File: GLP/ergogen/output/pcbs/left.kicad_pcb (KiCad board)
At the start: 2 copper layers, 138.8 x 106.7 mm, 66 parts

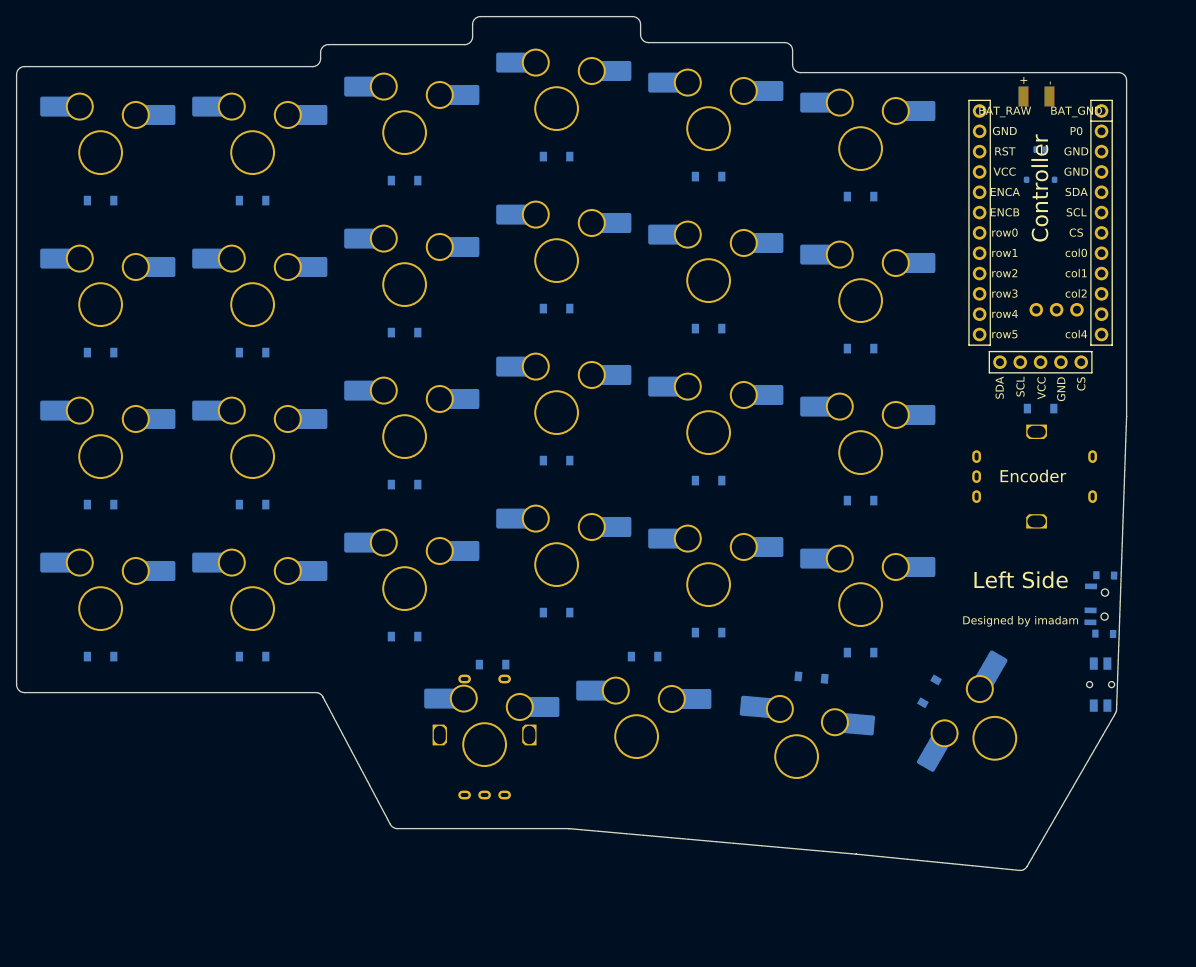
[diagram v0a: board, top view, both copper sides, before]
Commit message: er i lied
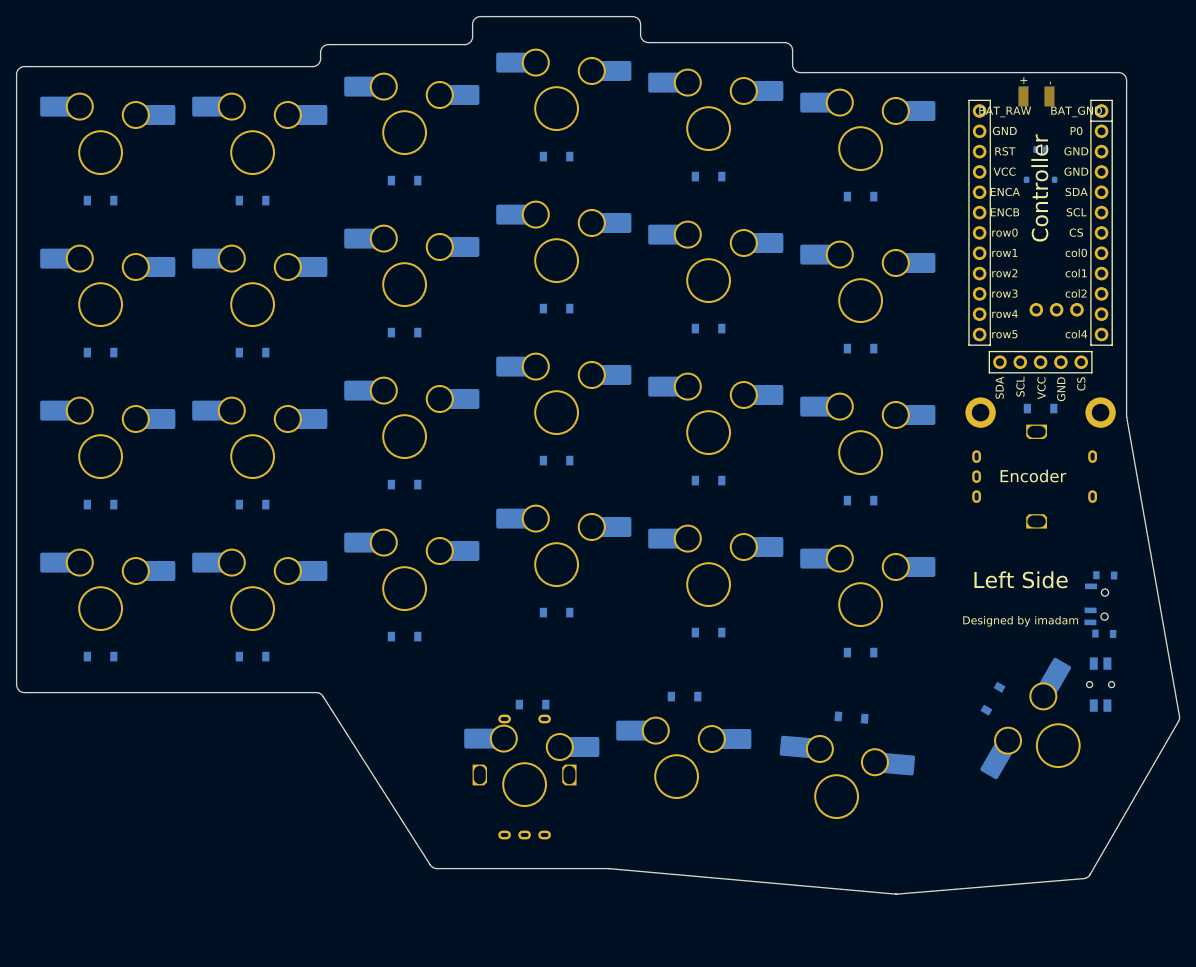
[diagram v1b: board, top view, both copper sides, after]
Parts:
- added H1: , ceoloide:mounting_hole_plated, F.Cu at (160.0, 106.5)
- added H2: , ceoloide:mounting_hole_plated, F.Cu at (175.0, 106.5)
- moved D28 7.99 mm to (161.6, 142.3)
- moved S28 7.99 mm to (169.7, 148.1)
- moved D25 7.07 mm to (104.0, 143.0)
- moved D26 7.07 mm to (123.0, 142.0)
- moved D27 7.07 mm to (143.9, 144.6)
- moved RE2 7.07 mm to (103.0, 151.8)
- moved S25 7.07 mm to (103.0, 153.0)
- moved S26 7.07 mm to (122.0, 152.0)
- moved S27 7.07 mm to (142.0, 154.5)
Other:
- board size 138.8 x 106.7 mm -> 145.4 x 109.7 mm
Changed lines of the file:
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@@
   (title_block
     (title "left")
-    (date "2025-04-06")
+    (date "2025-04-07")
     (rev "v1.0.0")
     (company "Unknown")
@@
   (footprint "ceoloide:switch_gateron_ks27_ks33"
     (layer "B.Cu")
-    (at 98 148 180)
+    (at 103 153 180)
     (property "Reference" "S25"
       (at 0 8.8 180)
@@
   (footprint "ceoloide:switch_gateron_ks27_ks33"
     (layer "B.Cu")
-    (at 117 147 180)
+    (at 122 152 180)
     (property "Reference" "S26"
       (at 0 8.8 180)
@@
   (footprint "ceoloide:switch_gateron_ks27_ks33"
     (layer "B.Cu")
-    (at 137 149.5 175)
+    (at 142 154.5 175)
     (property "Reference" "S27"
       (at 0 8.8 175)
@@
   (footprint "ceoloide:switch_gateron_ks27_ks33"
     (layer "B.Cu")
-    (at 161.777353 147.2132953 240)
+    (at 169.71036569999998 148.1331683 240)
     (property "Reference" "S28"
       (at 0 8.8 240)
@@
     (footprint "ceoloide:diode_tht_sod123"
         (layer "B.Cu")
-        (at 99 138 0)
+        (at 104 143 0)
         (property "Reference" "D25"
             (at 0 0 0)
@@
     (footprint "ceoloide:diode_tht_sod123"
         (layer "B.Cu")
-        (at 118 137 0)
+        (at 123 142 0)
         (property "Reference" "D26"
             (at 0 0 0)
@@
     (footprint "ceoloide:diode_tht_sod123"
         (layer "B.Cu")
-        (at 138.8677521 139.6252088 -5)
+        (at 143.8677521 144.6252088 -5)
         (property "Reference" "D27"
             (at 0 0 -5)
@@
     (footprint "ceoloide:diode_tht_sod123"
         (layer "B.Cu")
-        (at 153.617099 141.3472699 60)
+        (at 161.55011169999997 142.26714289999998 60)
         (property "Reference" "D28"
             (at 0 0 60)
@@
   (footprint "ceoloide:rotary_encoder_ec11_ec12"
     (layer "F.Cu")
-    (at 98 146.8 0)
+    (at 103 151.8 0)
     (property "Reference" "RE2"
       (at 0 -8.5)
@@
   )
   (gr_text "Bottom"
-    (at 136.4770655 155.4771682 -5)
+    (at 141.4770655 160.4771682 -5)
     (layer "B.SilkS" knockout)
     (effects
@@
       )
     )
+  )
+  (footprint "ceoloide:mounting_hole_plated"
+    (layer "F.Cu")
+    (at 160 106.5 0)
+    (property "Reference" "H1"
+      (at 0 3 0)
+      (layer "F.SilkS")
+      hide
+      (effects (font (size 1 1) (thickness 0.15)))
+    )
+    (pad "" thru_hole circle (at 0 0 0) (size 3.8000000000000003 3.8000000000000003) (drill 2.2) (layers "*.Cu" "*.Mask"))
+    (fp_circle (center 0 0) (end -2.1500000000000004 0) (layer "F.CrtYd") (stroke (width 0.05) (type solid)) (fill none))
+    (fp_circle (center 0 0) (end -2.1500000000000004 0) (layer "B.CrtYd") (stroke (width 0.05) (type solid)) (fill none))
+  )
+  (footprint "ceoloide:mounting_hole_plated"
+    (layer "F.Cu")
+    (at 175 106.5 0)
+    (property "Reference" "H2"
+      (at 0 3 0)
+      (layer "F.SilkS")
+      hide
+      (effects (font (size 1 1) (thickness 0.15)))
+    )
+    (pad "" thru_hole circle (at 0 0 0) (size 3.8000000000000003 3.8000000000000003) (drill 2.2) (layers "*.Cu" "*.Mask"))
+    (fp_circle (center 0 0) (end -2.1500000000000004 0) (layer "F.CrtYd") (stroke (width 0.05) (type solid)) (fill none))
+    (fp_circle (center 0 0) (end -2.1500000000000004 0) (layer "B.CrtYd") (stroke (width 0.05) (type solid)) (fill none))
   )
   (gr_line (start 39.5 140.51) (end 39.5 64.24) (layer Edge.Cuts) (stroke (width 0.15) (type default)))
@@
 (gr_line (start 136.5 61.24) (end 136.5 63.01) (layer Edge.Cuts) (stroke (width 0.15) (type default)))
 (gr_line (start 137.49 64) (end 177.26 64) (layer Edge.Cuts) (stroke (width 0.15) (type default)))
-(gr_line (start 178.25 106.98304477713282) (end 178.25 64.99) (layer Edge.Cuts) (stroke (width 0.15) (type default)))
-(gr_line (start 178.249419298365 107.01694732484975) (end 176.99510974489652 143.62299453267315) (layer Edge.Cuts) (stroke (width 0.15) (type default)))
-(gr_line (start 176.86305555803136 144.08409196503845) (end 165.80615268800693 163.23520942658655) (layer Edge.Cuts) (stroke (width 0.15) (type default)))
-(gr_line (start 164.85076974921034 163.7253452437892) (end 144.47054179145226 161.6975779835782) (layer Edge.Cuts) (stroke (width 0.15) (type default)))
-(gr_line (start 144.46018222869026 161.69660218659897) (end 108.54374262754885 158.5038884057367) (layer Edge.Cuts) (stroke (width 0.15) (type default)))
-(gr_line (start 87.09606054117646 158.5) (end 108.45608436301427 158.5) (layer Edge.Cuts) (stroke (width 0.15) (type default)))
-(gr_line (start 86.22111054608999 157.9732088092811) (end 77.77888945391003 142.02679119071894) (layer Edge.Cuts) (stroke (width 0.15) (type default)))
-(gr_line (start 40.49 141.5) (end 76.90393945882354 141.5) (layer Edge.Cuts) (stroke (width 0.15) (type default)))
+(gr_line (start 178.25 106.91330563065048) (end 178.25 64.99) (layer Edge.Cuts) (stroke (width 0.15) (type default)))
+(gr_line (start 178.26506800524558 107.08537446037167) (end 184.85701419664065 144.43496650770498) (layer Edge.Cuts) (stroke (width 0.15) (type default)))
+(gr_line (start 184.73944731338625 145.10203531750773) (end 173.67873709901966 164.25974729286952) (layer Edge.Cuts) (stroke (width 0.15) (type default)))
+(gr_line (start 172.90327558014778 164.75135351340012) (end 149.55016624203031 166.69002289360108) (layer Edge.Cuts) (stroke (width 0.15) (type default)))
+(gr_line (start 149.3806043848676 166.68952828725241) (end 113.54374262754898 163.5038884057367) (layer Edge.Cuts) (stroke (width 0.15) (type default)))
+(gr_line (start 92.04345643636363 163.5) (end 113.4560843630144 163.5) (layer Edge.Cuts) (stroke (width 0.15) (type default)))
+(gr_line (start 91.20823156106951 163.04150673882353) (end 77.7917684389305 141.9584932611765) (layer Edge.Cuts) (stroke (width 0.15) (type default)))
+(gr_line (start 40.49 141.5) (end 76.95654356363637 141.5) (layer Edge.Cuts) (stroke (width 0.15) (type default)))
 (gr_arc (start 40.49 63.24999999999999) (mid 39.7899643 63.539964299999994) (end 39.5 64.24) (layer Edge.Cuts) (stroke (width 0.15) (type default)))
 (gr_arc (start 76.51 63.25) (mid 77.2100357 62.9600357) (end 77.5 62.26) (layer Edge.Cuts) (stroke (width 0.15) (type default)))
@@
 (gr_arc (start 136.5 63.01) (mid 136.7899643 63.7100357) (end 137.49 64) (layer Edge.Cuts) (stroke (width 0.15) (type default)))
 (gr_arc (start 178.25 64.99) (mid 177.9600357 64.2899643) (end 177.26 63.99999999999999) (layer Edge.Cuts) (stroke (width 0.15) (type default)))
-(gr_arc (start 178.2494193 107.01694727713281) (mid 178.24985479999998 106.99999847713282) (end 178.25 106.98304477713282) (layer Edge.Cuts) (stroke (width 0.15) (type default)))
-(gr_arc (start 176.8630555465315 144.08409198495713) (mid 176.9574287465315 143.86166138495713) (end 176.9951097465315 143.62299458495713) (layer Edge.Cuts) (stroke (width 0.15) (type default)))
-(gr_arc (start 164.8507697765069 163.7253452465051) (mid 165.4006839765069 163.6210554465051) (end 165.8061527765069 163.2352094465051) (layer Edge.Cuts) (stroke (width 0.15) (type default)))
-(gr_arc (start 144.47054176415568 161.6975779808623) (mid 144.46536326415568 161.69707648086228) (end 144.46018216415567 161.6966021808623) (layer Edge.Cuts) (stroke (width 0.15) (type default)))
-(gr_arc (start 108.54374266301427 158.50388840000002) (mid 108.49995666301427 158.5009726) (end 108.45608436301427 158.5) (layer Edge.Cuts) (stroke (width 0.15) (type default)))
-(gr_arc (start 86.22111054117646 157.97320879999998) (mid 86.58541234117645 158.3581381) (end 87.09606054117646 158.49999989999998) (layer Edge.Cuts) (stroke (width 0.15) (type default)))
-(gr_arc (start 77.77888945882354 142.02679120000002) (mid 77.41458765882355 141.6418619) (end 76.90393945882354 141.50000010000002) (layer Edge.Cuts) (stroke (width 0.15) (type default)))
+(gr_arc (start 178.25 106.91330563065048) (mid 178.2537742 106.99966933065049) (end 178.265068 107.08537443065049) (layer Edge.Cuts) (stroke (width 0.15) (type default)))
+(gr_arc (start 184.73944730188623 145.1020353374263) (mid 184.85705570188622 144.77886843742627) (end 184.85701410188622 144.43496653742628) (layer Edge.Cuts) (stroke (width 0.15) (type default)))
+(gr_arc (start 172.90327558751966 164.75135351278814) (mid 173.35144328751966 164.60088391278813) (end 173.67873708751966 164.25974731278814) (layer Edge.Cuts) (stroke (width 0.15) (type default)))
+(gr_arc (start 149.38060434940223 166.68952829298908) (mid 149.4653746494022 166.6934124929891) (end 149.55016624940222 166.6900228929891) (layer Edge.Cuts) (stroke (width 0.15) (type default)))
+(gr_arc (start 113.5437426630144 163.50388840000002) (mid 113.4999566630144 163.5009726) (end 113.4560843630144 163.5) (layer Edge.Cuts) (stroke (width 0.15) (type default)))
+(gr_arc (start 91.20823153636363 163.04150669999999) (mid 91.56705933636363 163.37783969999998) (end 92.04345643636363 163.5) (layer Edge.Cuts) (stroke (width 0.15) (type default)))
+(gr_arc (start 77.79176846363637 141.95849330000001) (mid 77.43294066363637 141.62216030000002) (end 76.95654356363637 141.5) (layer Edge.Cuts) (stroke (width 0.15) (type default)))
 (gr_arc (start 39.5 140.51) (mid 39.7899643 141.2100357) (end 40.49 141.5) (layer Edge.Cuts) (stroke (width 0.15) (type default)))
 )

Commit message: ok
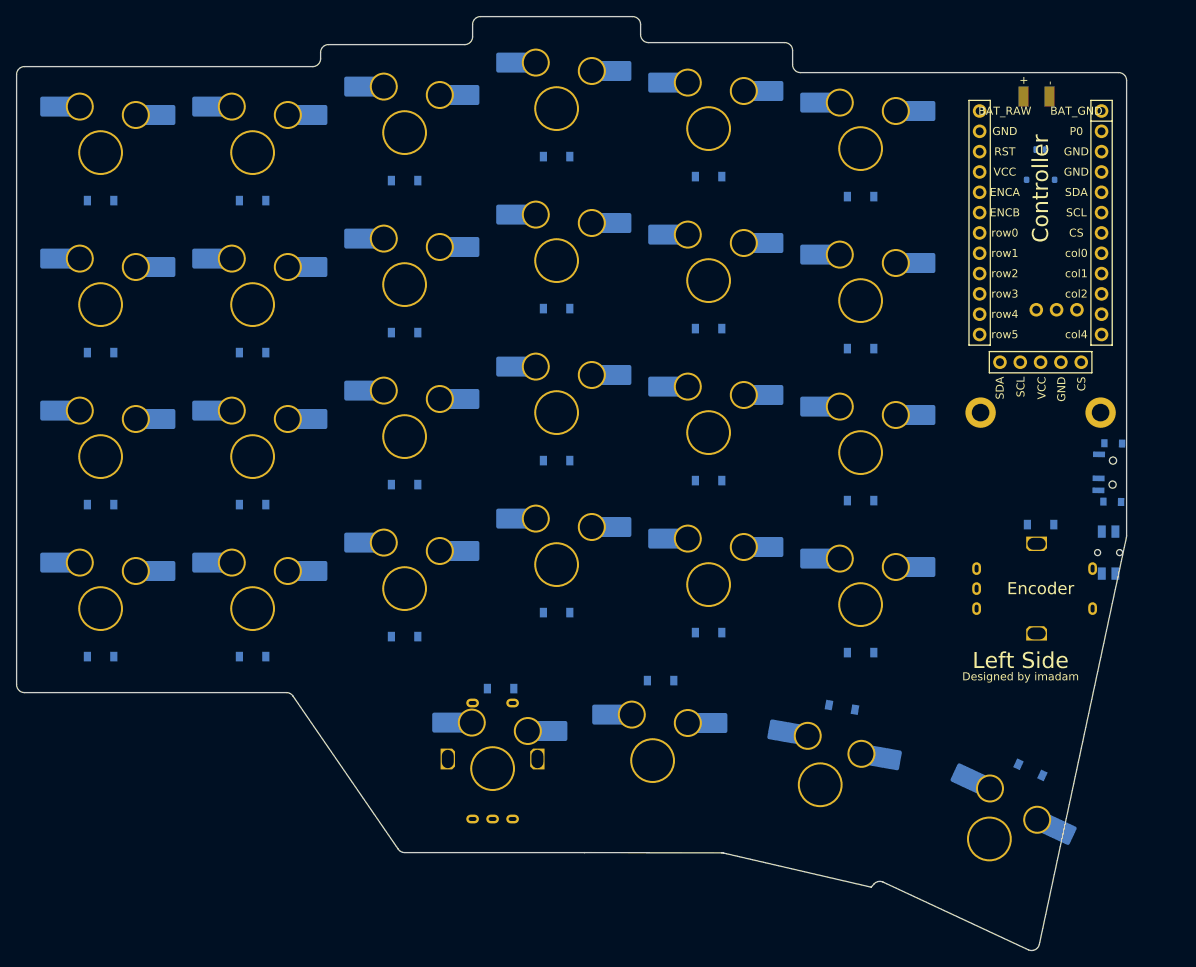
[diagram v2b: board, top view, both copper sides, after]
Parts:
- moved PWR1 16.5 mm to (176.5, 114.0)
- moved RST1 16.5 mm to (176.0, 124.0)
- moved D29 14.5 mm to (167.5, 120.5)
- moved S28 14.5 mm to (161.1, 159.8), turned to 155 degrees
- moved RE1 14.0 mm to (167.0, 128.5)
- moved D28 10.0 mm to (166.2, 151.2), turned to -25 degrees
- moved D25 4.47 mm to (100.0, 141.0)
- moved RE2 4.47 mm to (99.0, 149.8)
- moved S25 4.47 mm to (99.0, 151.0)
- moved D26 3.61 mm to (120.0, 140.0)
- moved S26 3.61 mm to (119.0, 150.0)
- moved S27 2.52 mm to (140.0, 153.0), turned to 170 degrees
- moved D27 1.75 mm to (142.7, 143.3), turned to -10 degrees
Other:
- board size 145.4 x 109.7 mm -> 138.8 x 116.7 mm
